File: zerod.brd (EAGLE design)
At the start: 82.2 x 80 mm, 38 parts, among them IC1 NE5532N, IC2 LM3914N, Q1 2N3906

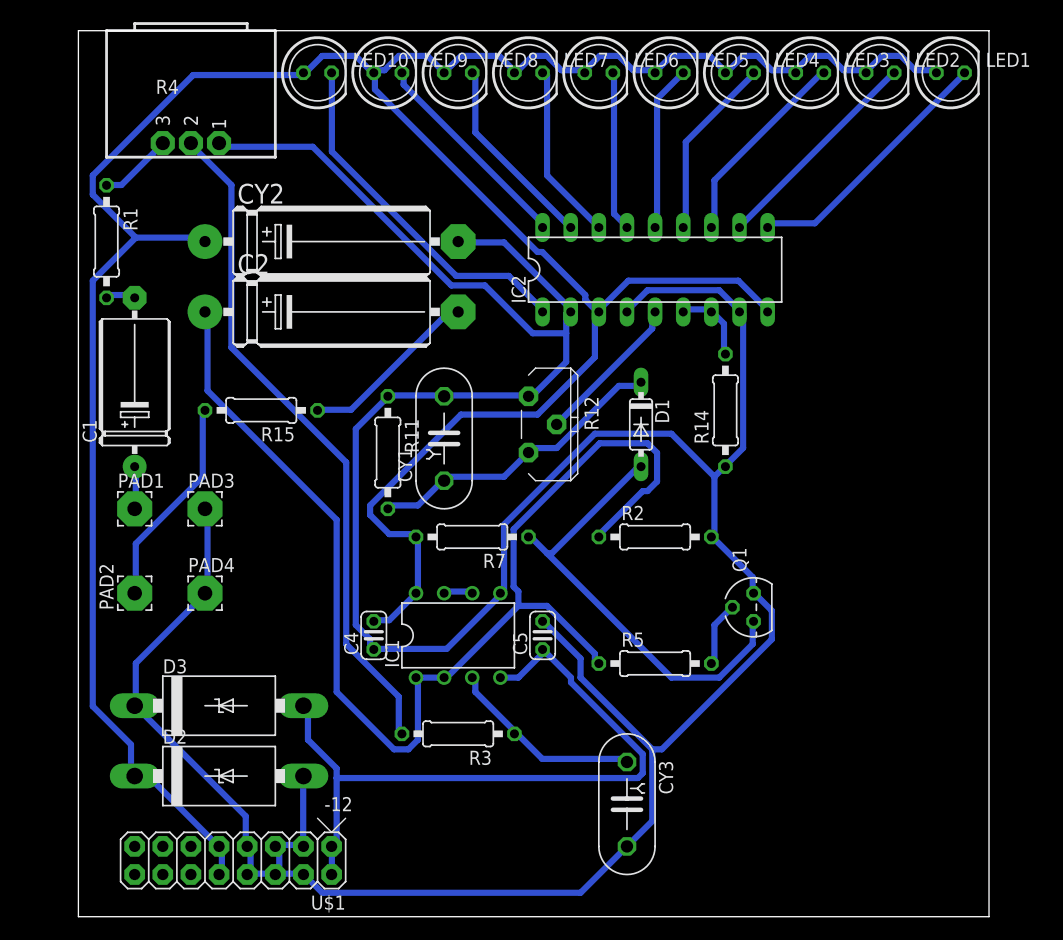
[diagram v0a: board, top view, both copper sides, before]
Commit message: redid layout
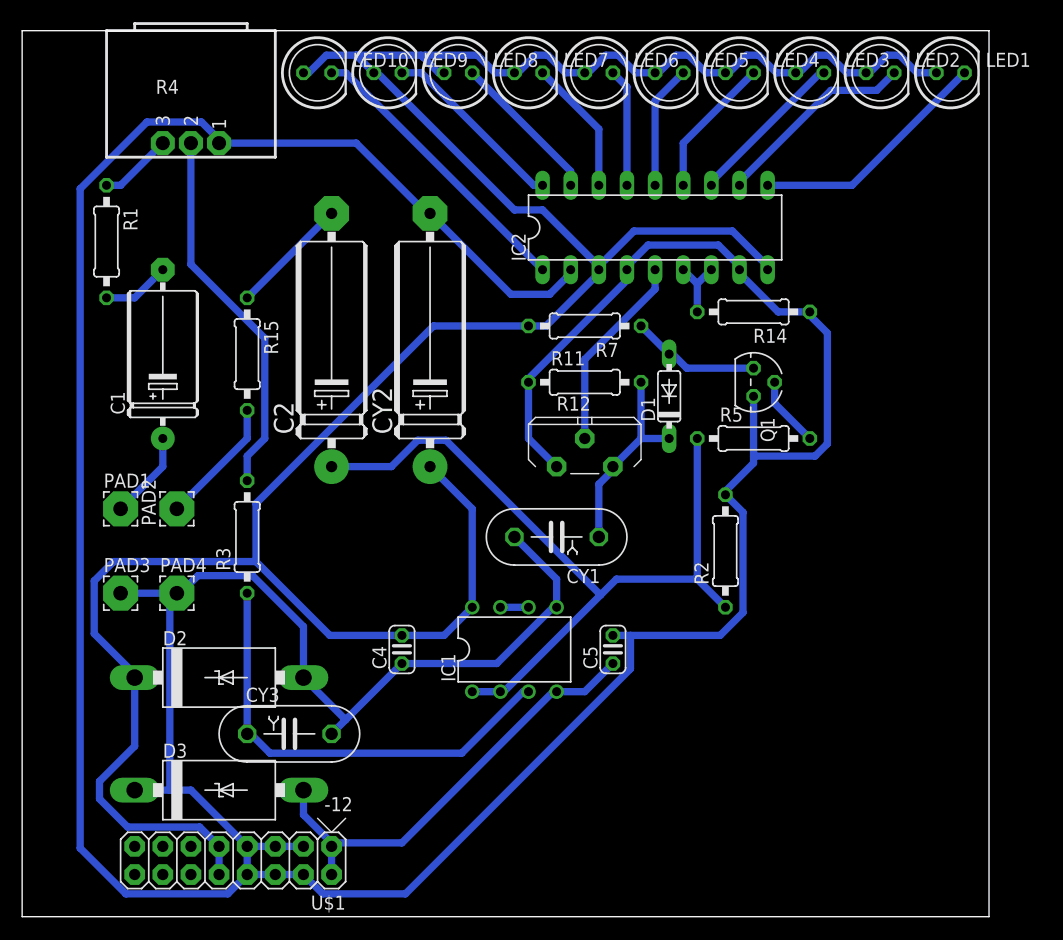
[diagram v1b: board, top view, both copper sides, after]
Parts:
- moved CY3 31.1 mm to (19.1, 16.5), turned to 0 degrees
- moved R3 26.1 mm to (15.2, 34.3), turned to 90 degrees
- moved R5 22.2 mm to (61.0, 43.2)
- moved R7 21.6 mm to (45.7, 53.3)
- moved Q1 20.3 mm to (61.0, 48.3), turned to 270 degrees
- moved R11 18.9 mm to (45.7, 48.3), turned to 0 degrees
- moved CY1 13.5 mm to (43.2, 34.3), turned to 180 degrees
- moved CY2 12.6 mm to (31.8, 52.1), turned to 90 degrees
- moved PAD3 10.8 mm to (3.81, 29.2)
- moved R14 9.25 mm to (61.0, 54.6), turned to 180 degrees
- moved D2 8.89 mm to (12.7, 21.6)
- moved PAD2 8.52 mm to (8.89, 36.8)
- moved D3 7.62 mm to (12.7, 11.4)
- moved C5 6.48 mm to (48.3, 24.1)
- moved R2 6.48 mm to (58.4, 33.0), turned to 90 degrees
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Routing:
- net GNDA: track 316.4 -> 375.0 mm
- net N$5: track 110.2 -> 71.9 mm
- net N$15: track 40.5 -> 11.7 mm
- net N$7: track 61.2 -> 33.9 mm
- net -12V: track 64.7 -> 40.9 mm
- net N$6: track 18.0 -> 41.1 mm
- net +12V: track 264.4 -> 253.3 mm
- net N$12: track 27.7 -> 18.1 mm
- net N$8: track 19.1 -> 11.5 mm
- net N$23: track 32.2 -> 26.4 mm
- net N$3: track 16.4 -> 10.8 mm
- net N$1: track 3.89 -> 7.93 mm
- net N$10: track 13.9 -> 17.9 mm
- net N$20: track 16.1 -> 12.3 mm
- net N$21: track 17.7 -> 13.8 mm
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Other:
- board size 82.2 x 80 mm -> 87.3 x 80 mm
